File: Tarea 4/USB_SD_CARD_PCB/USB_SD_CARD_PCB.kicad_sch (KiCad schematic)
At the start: 17 parts, among them J1 PZ254R-12-16P, U1 MT9700-N

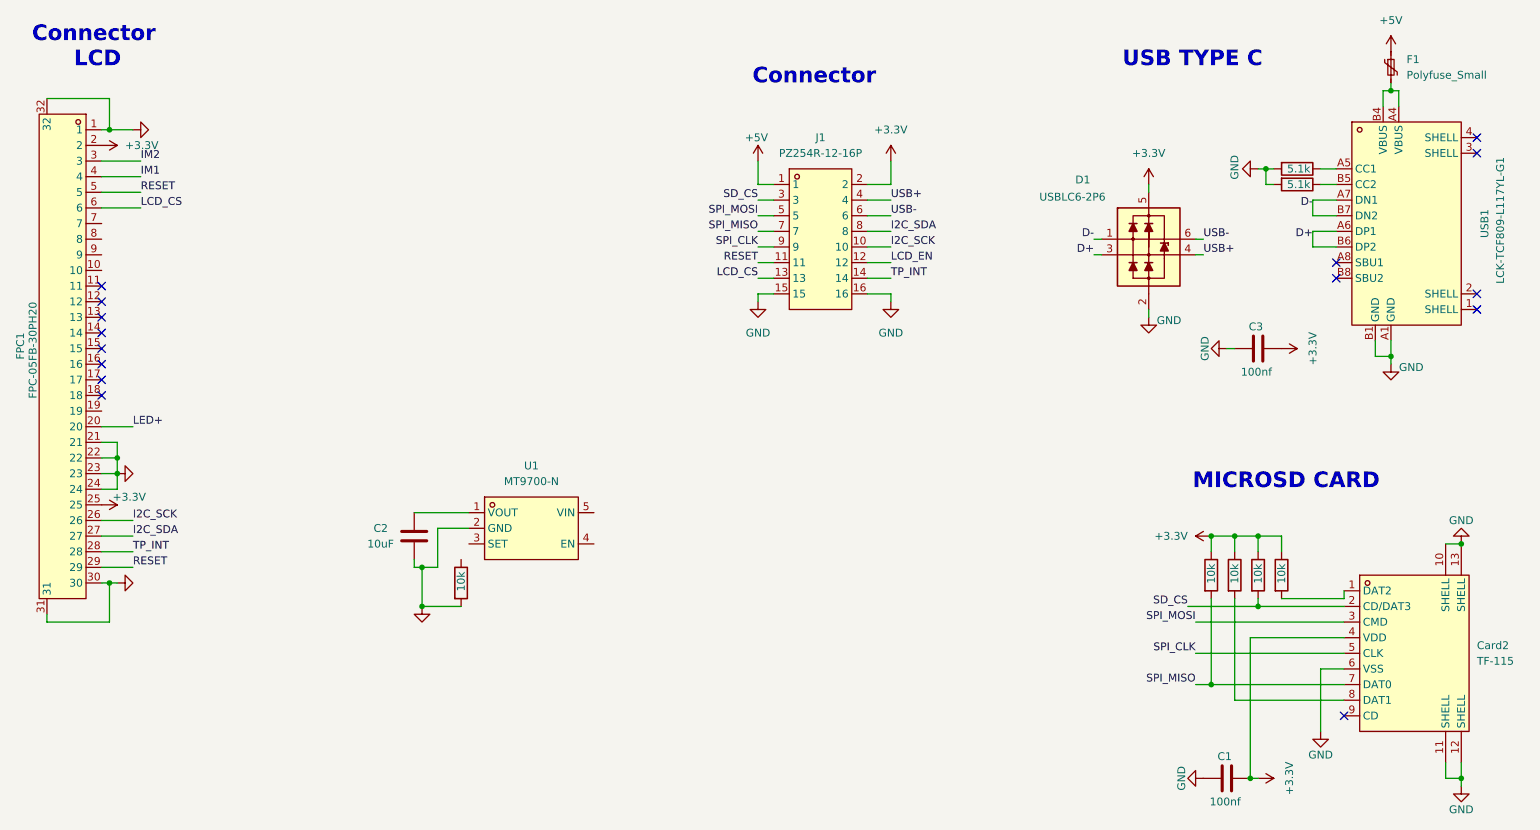
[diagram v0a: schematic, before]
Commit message: Actualizacion 18/04/26
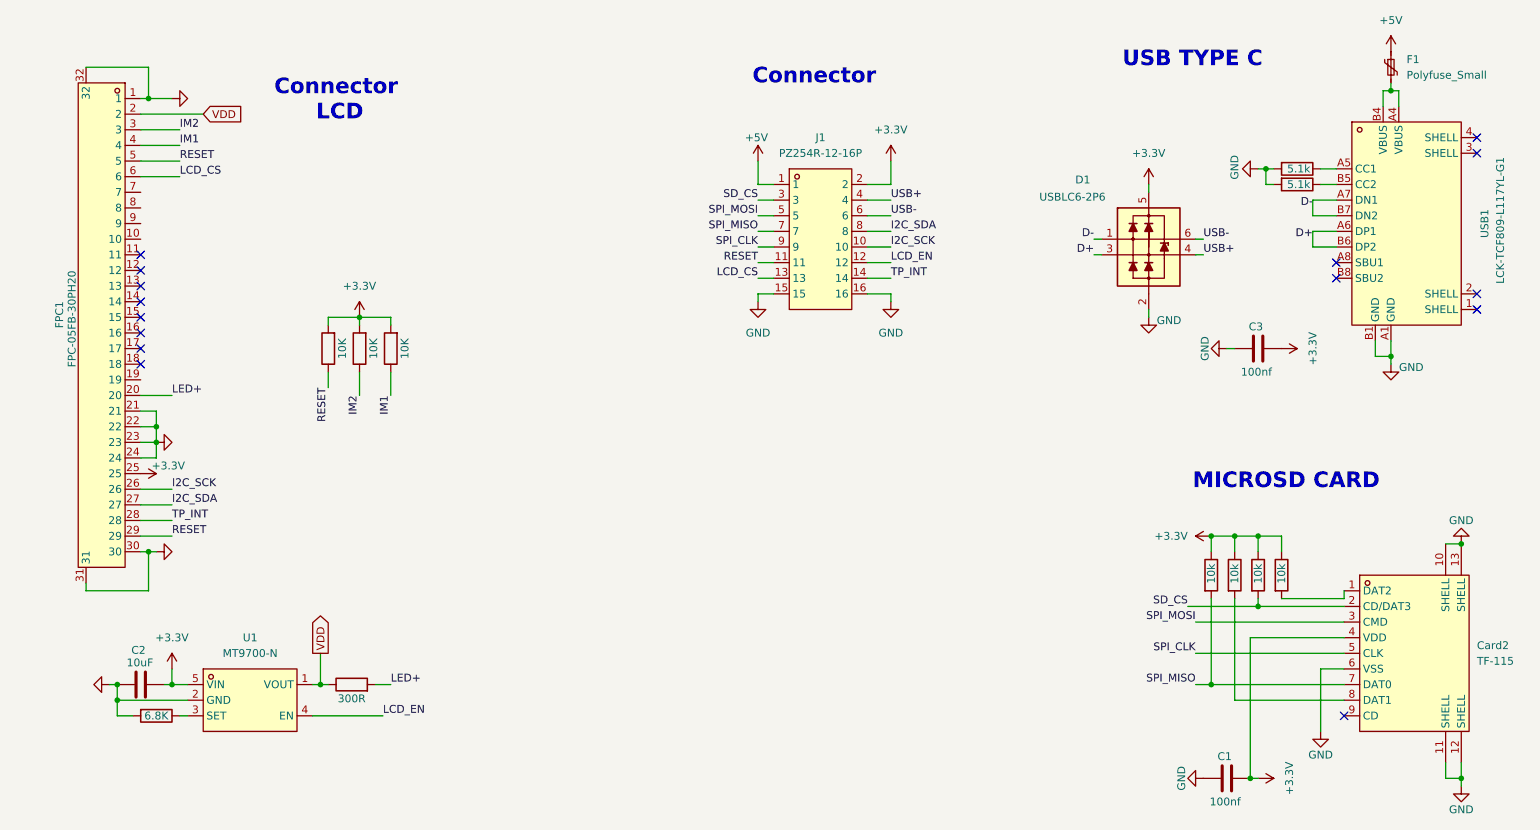
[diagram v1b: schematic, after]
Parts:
- added R10, R11, R9: 10K, PCM_Resistor_SMD_AKL:R_0603_1608Metric, symbol Device:R
- added R8: 300R, PCM_Resistor_SMD_AKL:R_0603_1608Metric, symbol Device:R
- C2: footprint Capacitor_SMD_AKL:C_0603_1608Metric -> Capacitor_SMD:C_0201_0603Metric
- R3, R4, R5, R6: footprint Resistor_SMD:R_0805_2012Metric -> PCM_Resistor_SMD_AKL:R_0603_1608Metric
- R7: value 10k -> 6.8K; footprint Resistor_SMD:R_0805_2012Metric -> PCM_Resistor_SMD_AKL:R_0603_1608Metric
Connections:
- net +3.3V: now also C2.1, U1.5 (VIN), R10.2, R11.2, R9.2; no longer FPC1.2
- net IM1: now also R11.1
- net IM2: now also R10.1
- net LCD_EN: now also U1.4 (EN)
- net LED+: now also R8.2
- net RESET: now also R9.1
- net VDD: now reaches U1.1 (VOUT)
- net VDD: now also FPC1.2, R8.1; no longer C2.1
- net at U1.3 (SET): now also R7.1
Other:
- moved on the sheet: C2, FPC1, U1
